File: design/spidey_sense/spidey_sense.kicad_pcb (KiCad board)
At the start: 2 copper layers, 60.8 x 39 mm, 27 parts, among them J1 Screw_Terminal_01x08, J2 Screw_Terminal_01x08, J3 Screw_Terminal_01x08, J4 Screw_Terminal_01x08, J5 Screw_Terminal_01x08, U1 LTC2984, U2 LM2931-5.0_SO8

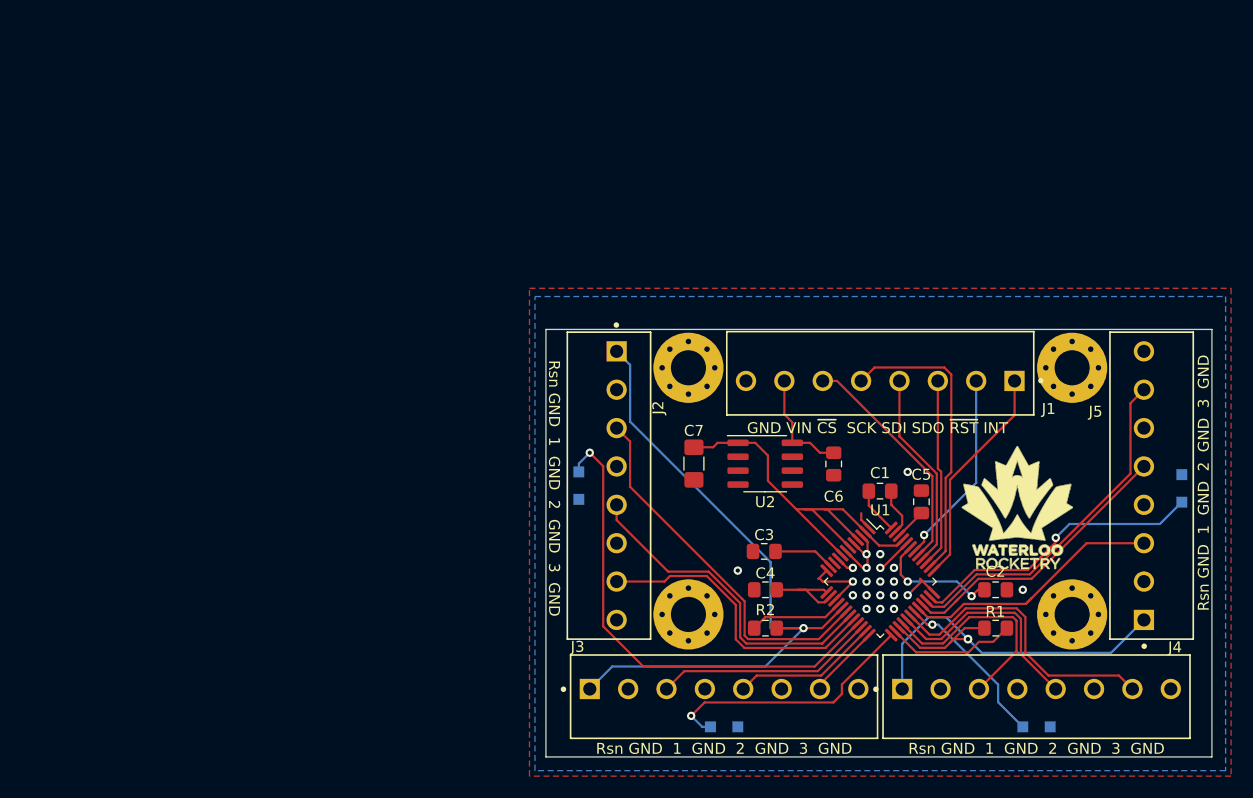
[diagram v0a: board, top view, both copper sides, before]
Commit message: Organized spidey_sense
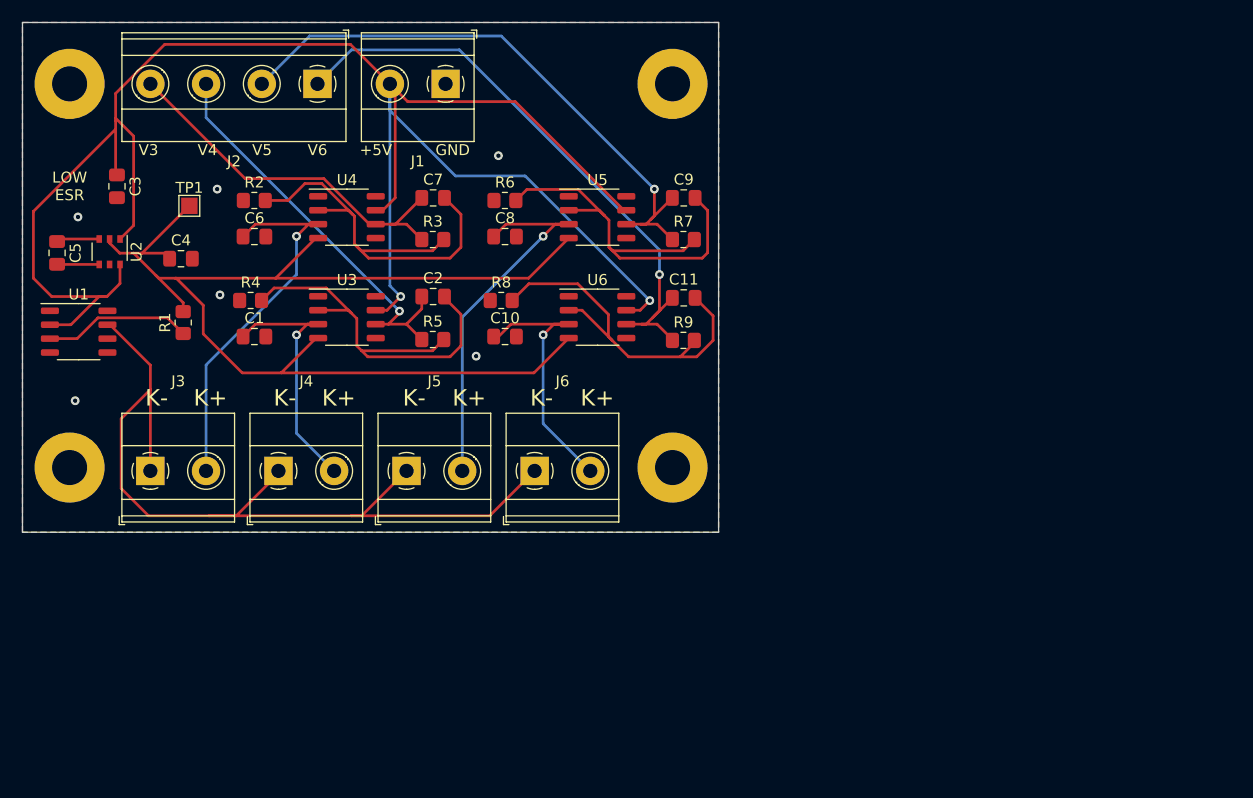
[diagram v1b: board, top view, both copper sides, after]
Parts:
- removed D1, D2, D3, D4: D, Diode_SMD:D_SOD-323_HandSoldering
- removed G***: LOGO, footprints:spider_man
- removed G*** (x2): LOGO, footprints:logo
- removed the REF** at (142.2, 115.0)
- removed the REF** at (142.2, 92.5)
- removed the REF** at (107.2, 92.5)
- removed the REF** at (107.2, 115.0)
- added C10: 0.1uF, Capacitor_SMD:C_0805_2012Metric_Pad1.18x1.45mm_HandSolder, F.Cu at (90.5, 89.6)
- added C11: 0.1uF, Capacitor_SMD:C_0805_2012Metric_Pad1.18x1.45mm_HandSolder, F.Cu at (106.8, 86.1)
- added C8: 0.1uF, Capacitor_SMD:C_0805_2012Metric_Pad1.18x1.45mm_HandSolder, F.Cu at (90.5, 80.5)
- added C9: 0.1uF, Capacitor_SMD:C_0805_2012Metric_Pad1.18x1.45mm_HandSolder, F.Cu at (106.8, 77.0)
- added J6: Thermocouple_Terminal, TerminalBlock_Phoenix:TerminalBlock_Phoenix_MKDS-1,5-2-5.08_1x02_P5.08mm_Horizontal, F.Cu at (93.2, 101.9)
- added R3: 17.3kΩ, Resistor_SMD:R_0805_2012Metric_Pad1.20x1.40mm_HandSolder, F.Cu at (83.9, 80.8)
- added R4: 1kΩ, Resistor_SMD:R_0805_2012Metric_Pad1.20x1.40mm_HandSolder, F.Cu at (67.3, 86.4)
- added R5: 17.3kΩ, Resistor_SMD:R_0805_2012Metric_Pad1.20x1.40mm_HandSolder, F.Cu at (83.9, 89.9)
- added R6: 1kΩ, Resistor_SMD:R_0805_2012Metric_Pad1.20x1.40mm_HandSolder, F.Cu at (90.5, 77.2)
- added R7: 17.3kΩ, Resistor_SMD:R_0805_2012Metric_Pad1.20x1.40mm_HandSolder, F.Cu at (106.8, 80.8)
- added R8: 1kΩ, Resistor_SMD:R_0805_2012Metric_Pad1.20x1.40mm_HandSolder, F.Cu at (90.2, 86.4)
- added R9: 17.3kΩ, Resistor_SMD:R_0805_2012Metric_Pad1.20x1.40mm_HandSolder, F.Cu at (106.8, 90.0)
- added REF**: MountingHole_3.2mm_M3_Pad, MountingHole:MountingHole_3.2mm_M3_Pad, F.Cu at (50.8, 66.6)
- added REF**: MountingHole_3.2mm_M3_Pad, MountingHole:MountingHole_3.2mm_M3_Pad, F.Cu at (105.8, 101.6)
- added REF**: MountingHole_3.2mm_M3_Pad, MountingHole:MountingHole_3.2mm_M3_Pad, F.Cu at (50.8, 101.6)
- added REF**: MountingHole_3.2mm_M3_Pad, MountingHole:MountingHole_3.2mm_M3_Pad, F.Cu at (105.8, 66.6)
- added TP1: TestPoint, TestPoint:TestPoint_Pad_1.5x1.5mm, F.Cu at (61.7, 77.7)
- added U3: LT1001, Package_SO:SOP-8_3.9x4.9mm_P1.27mm, F.Cu at (76.1, 87.9)
- added U4: LT1001, Package_SO:SOP-8_3.9x4.9mm_P1.27mm, F.Cu at (76.1, 78.8)
- added U5: LT1001, Package_SO:SOP-8_3.9x4.9mm_P1.27mm, F.Cu at (99.0, 78.8)
- added U6: LT1001, Package_SO:SOP-8_3.9x4.9mm_P1.27mm, F.Cu at (99.0, 87.9)
- C1, C2: value 10uF -> 0.1uF; footprint Capacitor_SMD:C_0805_2012Metric_Pad1.15x1.40mm_HandSolder -> Capacitor_SMD:C_0805_2012Metric_Pad1.18x1.45mm_HandSolder
- C3: value 0.1uF -> 10uF; footprint Capacitor_SMD:C_0805_2012Metric_Pad1.15x1.40mm_HandSolder -> Capacitor_SMD:C_0805_2012Metric_Pad1.18x1.45mm_HandSolder
- C4: value 1uF -> 10uF; footprint Capacitor_SMD:C_0805_2012Metric_Pad1.15x1.40mm_HandSolder -> Capacitor_SMD:C_0805_2012Metric_Pad1.18x1.45mm_HandSolder
- C5: value 10uF -> 1uF; footprint Capacitor_SMD:C_0805_2012Metric_Pad1.15x1.40mm_HandSolder -> Capacitor_SMD:C_0805_2012Metric_Pad1.18x1.45mm_HandSolder
- C6: footprint Capacitor_SMD:C_0805_2012Metric_Pad1.15x1.40mm_HandSolder -> Capacitor_SMD:C_0805_2012Metric_Pad1.18x1.45mm_HandSolder
- C7: value 100uF -> 0.1uF; footprint Capacitor_SMD:C_1206_3216Metric_Pad1.42x1.75mm_HandSolder -> Capacitor_SMD:C_0805_2012Metric_Pad1.18x1.45mm_HandSolder
- J1: value Screw_Terminal_01x08 -> Input_Screw_Terminal; footprint footprints:Phoenix_Contact-1984675-0-0-0 -> TerminalBlock_Phoenix:TerminalBlock_Phoenix_MKDS-1,5-2-5.08_1x02_P5.08mm_Horizontal
- J2: value Screw_Terminal_01x08 -> Output_Screw_Terminal; footprint footprints:Phoenix_Contact-1984675-0-0-0 -> TerminalBlock_Phoenix:TerminalBlock_Phoenix_MKDS-1,5-4-5.08_1x04_P5.08mm_Horizontal
- J3, J4, J5: value Screw_Terminal_01x08 -> Thermocouple_Terminal; footprint footprints:Phoenix_Contact-1984675-0-0-0 -> TerminalBlock_Phoenix:TerminalBlock_Phoenix_MKDS-1,5-2-5.08_1x02_P5.08mm_Horizontal
- R1: value 10K -> 150kΩ; footprint Resistor_SMD:R_0805_2012Metric_Pad1.15x1.40mm_HandSolder -> Resistor_SMD:R_0805_2012Metric_Pad1.20x1.40mm_HandSolder
- R2: value 10K -> 1kΩ; footprint Resistor_SMD:R_0805_2012Metric_Pad1.15x1.40mm_HandSolder -> Resistor_SMD:R_0805_2012Metric_Pad1.20x1.40mm_HandSolder
- U1: value LTC2984 -> LT1025; footprint Package_QFP:LQFP-48_7x7mm_P0.5mm -> Package_SO:SOP-8_3.9x4.9mm_P1.27mm
- U2: value LM2931-5.0_SO8 -> LTC1983-5; footprint Package_SO:SOIC-8_3.9x4.9mm_P1.27mm -> Package_SO:TSOP-6_1.65x3.05mm_P0.95mm
- moved C5 82.0 mm to (49.7, 82.0), turned to -90 degrees
- moved R1 79.2 mm to (61.2, 88.4), turned to 90 degrees
- moved U1 76.6 mm to (51.6, 89.2), turned to 0 degrees
- moved J4 72.2 mm to (69.8, 101.9)
- moved J5 68.0 mm to (81.5, 101.9), turned to 0 degrees
- moved C3 67.8 mm to (55.1, 75.9), turned to -90 degrees
- moved U2 62.8 mm to (54.4, 81.9), turned to -90 degrees
- moved C4 61.3 mm to (61.0, 82.5), turned to 0 degrees
- moved R2 60.8 mm to (67.6, 77.2)
- moved C1 58.8 mm to (67.7, 89.6)
- moved C2 57.9 mm to (84.0, 86.0)
- moved C6 56.8 mm to (67.7, 80.5), turned to 0 degrees
- moved J3 56.2 mm to (58.2, 101.9)
- moved J1 47.6 mm to (85.1, 66.6)
- moved J2 45.3 mm to (73.4, 66.6), turned to 180 degrees
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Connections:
- C1 pad 1: Net-(C1-Pad1) -> /Amplifier2/K+
- C1 pad 2: Net-(C1-Pad2) -> GND
- C2 pad 1: Net-(C2-Pad1) -> /Amplifier2/Vout
- C2 pad 2: GND -> Net-(C2-Pad2)
- C3 pad 1: Net-(C3-Pad1) -> +5V
- C4 pad 1: Net-(C4-Pad1) -> -5V
- C5 pad 2: GND -> Net-(C5-Pad2)
- C6 pad 1: Net-(C6-Pad1) -> /Amplifier1/K+
- C7 pad 1: +5V -> /Amplifier1/Vout
- C7 pad 2: GND -> Net-(C7-Pad2)
- J1 pad 1: Net-(J1-Pad1) -> GND
- J1 pad 2: Net-(J1-Pad2) -> +5V
- J2 pad 1: /Sheet60AF3A60/R_sense -> /Amplifier4/Vout
- J2 pad 2: GND -> /Amplifier3/Vout
- J2 pad 3: /Sheet60AF3A60/conn_1 -> /Amplifier2/Vout
- J2 pad 4: GND -> /Amplifier1/Vout
- J3 pad 1: /Sheet60AF3A60/R_sense -> /K-
- J3 pad 2: GND -> /Amplifier1/K+
- J4 pad 1: /sheet60B815B9/R_sense -> /K-
- J4 pad 2: GND -> /Amplifier2/K+
- J5 pad 1: /sheet60B815B9/R_sense -> /K-
- J5 pad 2: GND -> /Amplifier3/K+
- R1 pad 2: /sheet60B815B9/R_sense -> -5V
- R2 pad 1: Net-(R2-Pad1) -> GND
- R2 pad 2: /Sheet60AF3A60/R_sense -> Net-(C7-Pad2)
- U1 pad 1: GND -> unconnected-(U1-Pad1)
- U1 pad 3: GND -> Net-(R1-Pad1)
- U1 pad 4: +5V -> GND
- U1 pad 6: +5V -> unconnected-(U1-Pad6)
- U1 pad 7: GND -> /K-
- U1 pad 8: +5V -> unconnected-(U1-Pad8)
- U2 pad 2: GND -> -5V
- U2 pad 3: GND -> Net-(C5-Pad1)
- U2 pad 4: Net-(U2-Pad4) -> Net-(C5-Pad2)
- U2 pad 5: Net-(U2-Pad5) -> GND
- U2 pad 6: GND -> +5V
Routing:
- net +5V: track 40.4 -> 179.1 mm, vias 0 -> 2
- net -5V: track 0.00 -> 111.9 mm
- net /K-: track 0.00 -> 80.6 mm
- net /Sheet60AF3A60/R_sense: track 62.6 -> 0.00 mm, vias 1 -> 0
- net /Amplifier3/Vout: track 0.00 -> 55.0 mm, vias 0 -> 1
- net /Amplifier4/Vout: track 0.00 -> 54.9 mm, vias 0 -> 1
- net Net-(D1-Pad2): track 44.9 -> 0.00 mm, vias 1 -> 0
- net /sheet60B815B9/R_sense: track 40.9 -> 0.00 mm, vias 1 -> 0
- net Net-(C7-Pad2): track 0.00 -> 40.5 mm
- net Net-(C9-Pad2): track 0.00 -> 39.4 mm
- net Net-(C2-Pad2): track 0.00 -> 39.3 mm
- net /Amplifier2/Vout: track 0.00 -> 37.5 mm, vias 0 -> 1
- net Net-(C11-Pad2): track 0.00 -> 35.2 mm
- net /Amplifier3/K+: track 0.00 -> 34.6 mm, vias 0 -> 1
- net /Amplifier1/K+: track 0.00 -> 34.6 mm, vias 0 -> 1
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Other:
- board size 60.8 x 39 mm -> 63.5 x 46.5 mm
- net class Default removed
- rule pad_to_mask_clearance: 0.05 -> 0
- board text added: "+5V"
- board text added: "GND"
- board text added: "K+"
- board text added: "K-"
- board text added: "LOW ESR"
- board text added: "V3"
- board text added: "V4"
- board text added: "V5"
- board text added: "V6"
- board text removed: "GND VIN ~CS~ SCK SDI SDO ~RST~ INT"
- board text removed: "Rsn GND 1 GND 2 GND 3 GND"
- board text removed: "SPIdey Sense Z.Mears 2021-05-26"
